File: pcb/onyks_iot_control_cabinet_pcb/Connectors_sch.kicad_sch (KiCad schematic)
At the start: 5 parts, among them J1 Conn_01x04_Socket, J2 Screw_Terminal_01x02, J3 Conn_01x02_Socket, J5 Conn_01x04_Socket, J6 Conn_01x07_Socket

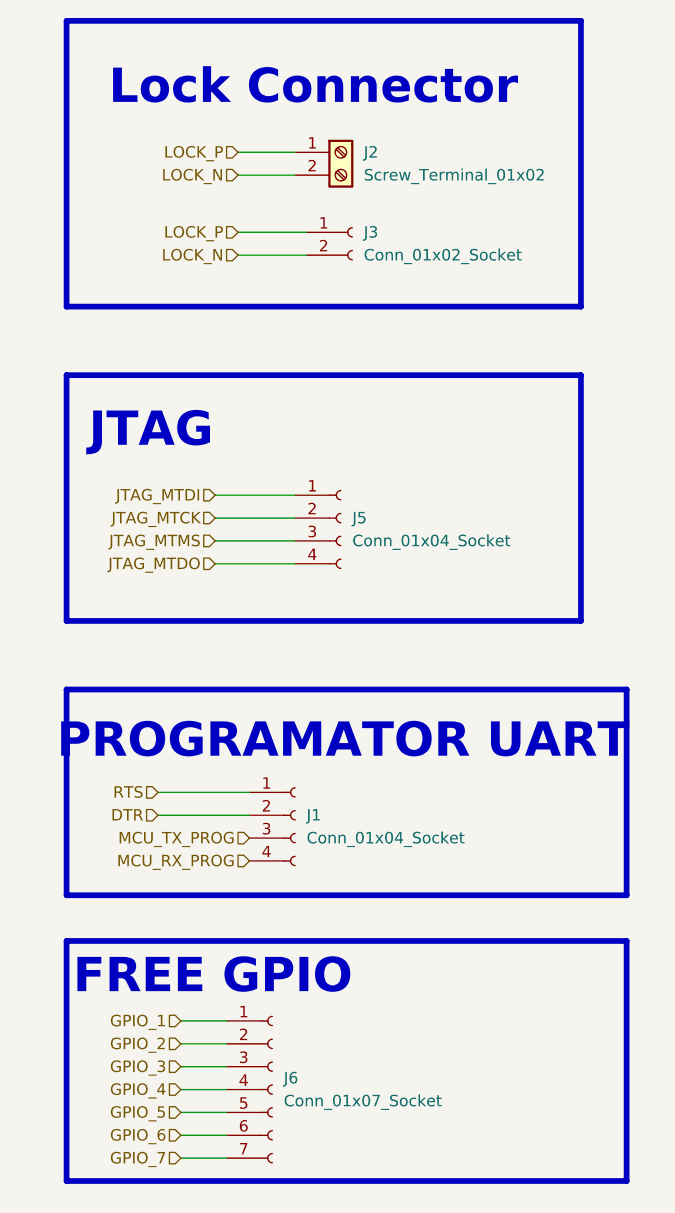
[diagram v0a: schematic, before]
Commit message: Fix the project; cleaning up the things
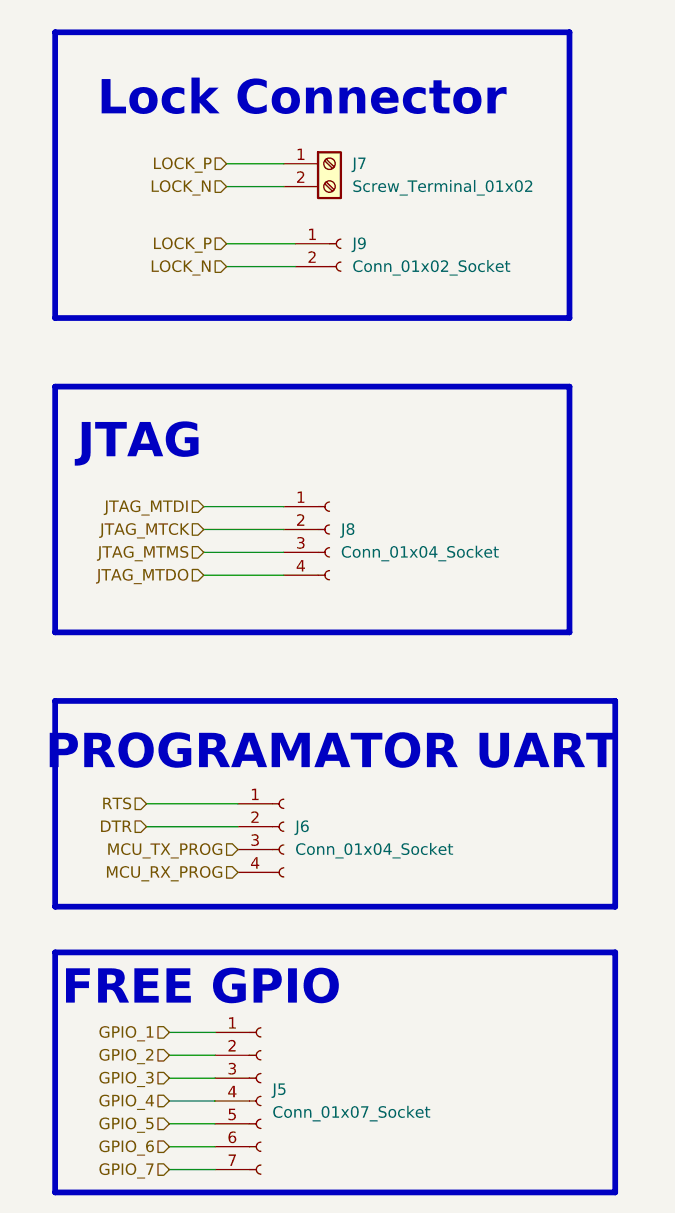
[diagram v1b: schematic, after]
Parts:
- removed J1, J5: Conn_01x04_Socket, symbol Connector:Conn_01x04_Socket
- removed J2: Screw_Terminal_01x02, symbol Connector:Screw_Terminal_01x02
- removed J3: Conn_01x02_Socket, symbol Connector:Conn_01x02_Socket
- removed J6: Conn_01x07_Socket, symbol Connector:Conn_01x07_Socket
- added J5: Conn_01x07_Socket, symbol Connector:Conn_01x07_Socket
- added J6, J8: Conn_01x04_Socket, symbol Connector:Conn_01x04_Socket
- added J7: Screw_Terminal_01x02, symbol Connector:Screw_Terminal_01x02
- added J9: Conn_01x02_Socket, symbol Connector:Conn_01x02_Socket
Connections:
- net DTR: now also J6.2 (Pin_2)
- net GPIO_1: now also J5.1 (Pin_1)
- net GPIO_2: now also J5.2 (Pin_2)
- net GPIO_3: now also J5.3 (Pin_3)
- net GPIO_4: now also J5.4 (Pin_4)
- net GPIO_5: now also J5.5 (Pin_5)
- net GPIO_6: now also J5.6 (Pin_6)
- net GPIO_7: now also J5.7 (Pin_7)
- net JTAG_MTCK: now also J8.2 (Pin_2)
- net JTAG_MTDI: now also J8.1 (Pin_1)
- net JTAG_MTDO: now also J8.4 (Pin_4)
- net JTAG_MTMS: now also J8.3 (Pin_3)
- net LOCK_N: now also J7.2 (Pin_2), J9.2 (Pin_2)
- net LOCK_P: now also J7.1 (Pin_1), J9.1 (Pin_1)
- net MCU_RX_PROG: now also J6.4 (Pin_4)
- net MCU_TX_PROG: now also J6.3 (Pin_3)
- net RTS: now also J6.1 (Pin_1)
